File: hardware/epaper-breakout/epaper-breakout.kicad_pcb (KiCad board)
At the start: 2 copper layers, 99.6 x 31.2 mm, 68 parts, among them J1 XF2M-3315-1A, J2 C10418, J3 Conn_02x06_Counter_Clockwise, J4 ED060SC4, Q1 IRLML6402, U1 MCP1700-3302E_SOT23, U2 LT1945, U3 LT1945, U5 ESP32-WROVER, U6 CH330N, U7 LM358, U8 74HC4094-normal, U9 MCP9700AT-ETT

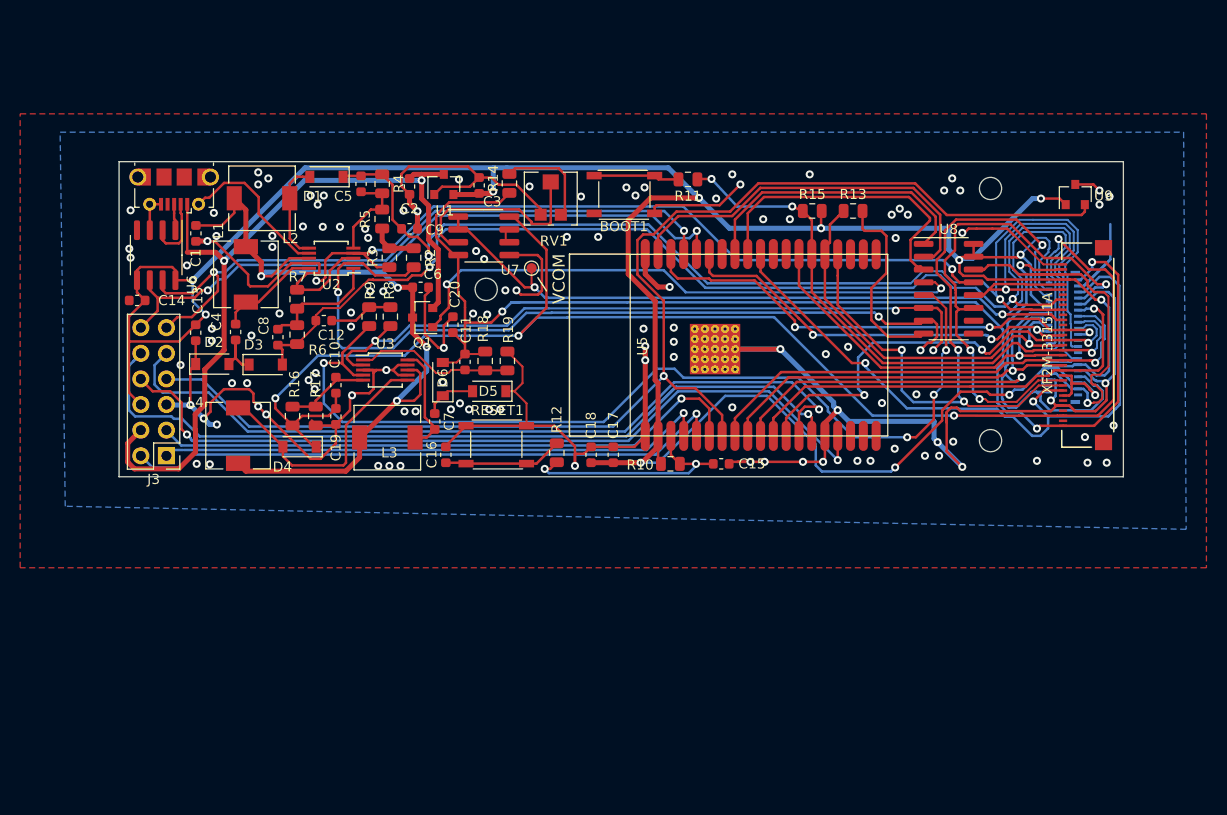
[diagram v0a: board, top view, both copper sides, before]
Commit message: WIP: partial routing
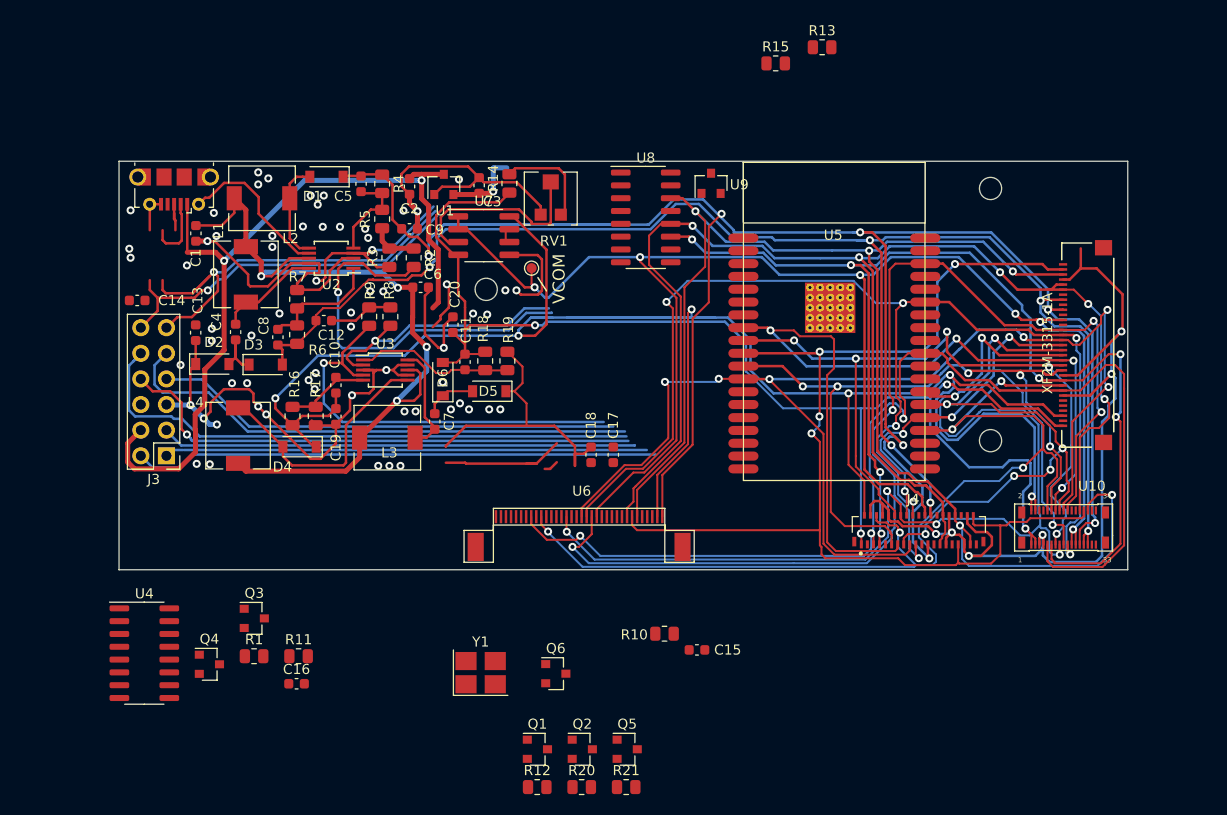
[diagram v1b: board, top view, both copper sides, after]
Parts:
- removed BOOT1: SW2, epaper-breakout:SW_TS-1187A
- removed RESET1: SW1, epaper-breakout:SW_TS-1187A
- added Q2: AO3401A, Package_TO_SOT_SMD:SOT-23, F.Cu at (70.9, 77.8)
- added Q3: MMBT3904, Package_TO_SOT_SMD:SOT-23, F.Cu at (38.4, 64.8)
- added Q4: MMBT3904, Package_TO_SOT_SMD:SOT-23, F.Cu at (34.0, 69.4)
- added Q5: AO3401A, Package_TO_SOT_SMD:SOT-23, F.Cu at (75.4, 77.8)
- added Q6: MMBT3904, Package_TO_SOT_SMD:SOT-23, F.Cu at (68.3, 70.3)
- added R1: 10k, Resistor_SMD:R_0805_2012Metric, F.Cu at (38.4, 68.6)
- added R20: 10k, Resistor_SMD:R_0805_2012Metric, F.Cu at (70.9, 81.5)
- added R21: 10k, Resistor_SMD:R_0805_2012Metric, F.Cu at (75.3, 81.5)
- added U10: ED060SC7, epaper-breakout:AXT334124, F.Cu at (118.6, 57.5)
- added U4: CH340G, Package_SO:SOIC-16_3.9x9.9mm_P1.27mm, F.Cu at (27.5, 68.3)
- added Y1: Crystal_GND2, Crystal:Crystal_SMD_3225-4Pin_3.2x2.5mm_HandSoldering, F.Cu at (60.9, 70.2)
- C13, C14: value 0.1uF -> 10pF
- C15, C16: value 1nF -> 0.1uF
- J4: moved to F.Cu
- Q1: value IRLML6402 -> MMBT3904
- R11: value 470 -> 10k
- R12: value 470 -> 1k
- U6: value CH330N -> ED060XC5; footprint Package_SO:SOIC-8_3.9x4.9mm_P1.27mm -> epaper-breakout:X05A20H34G
- moved R11 61.0 mm to (42.8, 68.6), turned to 0 degrees
- moved U6 49.3 mm to (70.6, 54.7), turned to 0 degrees
- moved Q1 44.3 mm to (66.5, 77.8), turned to 0 degrees
- moved U9 36.1 mm to (83.7, 21.7)
- moved R12 33.2 mm to (66.5, 81.5), turned to 0 degrees
- moved U8 30.9 mm to (77.2, 25.1)
- moved C16 27.1 mm to (42.6, 71.3), turned to 0 degrees
- moved J4 23.9 mm to (104.3, 56.1), turned to 0 degrees
- moved U5 22.8 mm to (95.9, 26.2), turned to 0 degrees
- moved C15 18.6 mm to (82.3, 67.9)
- moved R10 16.9 mm to (79.1, 66.3)
- moved R13 16.5 mm to (94.7, 8.20)
- moved R15 15.1 mm to (90.1, 9.80)
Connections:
- C1 pad 1: EPD_POWER -> SW_VIN
- C13 pad 1: /+3.3V -> Net-(C13-Pad1)
- C14 pad 1: /+3.3V -> GND
- C14 pad 2: GND -> Net-(C14-Pad2)
- C15 pad 1: GND -> /EN
- C15 pad 2: /EN -> GND
- C16 pad 1: GND -> /+3.3V
- C16 pad 2: Net-(C16-Pad2) -> GND
- C6 pad 1: EPD_POWER -> SW_VIN
- J1 pad 11: /+3.3V -> EPD_VDD
- J1 pad 30: /+3.3V -> EPD_VDD
- J1 pad 7: /+3.3V -> EPD_VDD
- J4 pad 10: /+3.3V -> EPD_VDD
- J4 pad 29: /+3.3V -> EPD_VDD
- J4 pad 30: /+3.3V -> EPD_VDD
- J4 pad 35: /+3.3V -> EPD_VDD
- J4 pad 36: /+3.3V -> EPD_VDD
- J4 pad 4: /+3.3V -> EPD_VDD
- J4 pad 8: /+3.3V -> EPD_VDD
- L1 pad 2: EPD_POWER -> SW_VIN
- L2 pad 2: EPD_POWER -> SW_VIN
- L3 pad 2: EPD_POWER -> SW_VIN
- L4 pad 2: EPD_POWER -> SW_VIN
- Q1 pad 1: /~SMPS_CTRL -> Net-(Q1-Pad1)
- Q1 pad 2: 5V -> GND
- Q1 pad 3: EPD_POWER -> Net-(Q1-Pad3)
- R11 pad 1: /EP_D3 -> Net-(Q4-Pad1)
- R11 pad 2: Net-(BOOT1-Pad2) -> /~RTS
- R12 pad 1: /EN -> Net-(Q1-Pad1)
- R12 pad 2: Net-(C16-Pad2) -> /SMPS_CTRL
- U2 pad 8: EPD_POWER -> SW_VIN
- U3 pad 8: EPD_POWER -> SW_VIN
- U6 pad 1: Net-(J2-Pad3) -> /-15V
- U6 pad 2: Net-(J2-Pad2) -> /-20V
- U6 pad 5: /+3.3V -> (no net)
- U6 pad 6: /USB_TXD -> EPD_VDD
- U6 pad 7: /USB_RXD -> GND
- U6 pad 8: /+3.3V -> /EP_CKH
- U8 pad 4: /~SMPS_CTRL -> /SMPS_CTRL
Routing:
- net /+3.3V: track 306.9 -> 8.42 mm, vias 13 -> 1
- net GND: track 368.8 -> 187.1 mm, vias 122 -> 62
- net /EP_STV: track 37.3 -> 139.0 mm, vias 1 -> 5
- net /+22V: track 115.5 -> 210.9 mm, vias 2 -> 7
- net EPD_VDD: track 0.00 -> 94.2 mm, vias 0 -> 6
- net /EP_MODE: track 46.7 -> 138.2 mm, vias 1 -> 5
- net SW_VIN: track 0.00 -> 81.7 mm, vias 0 -> 4
- net EPD_POWER: track 81.7 -> 0.00 mm, vias 4 -> 0
- net /A1: track 126.2 -> 46.3 mm, vias 1 -> 0
- net /EP_D6: track 41.9 -> 118.7 mm, vias 3 -> 6
- net /EP_D5: track 43.6 -> 117.2 mm, vias 3 -> 6
- net /EP_D7: track 48.5 -> 119.5 mm, vias 3 -> 5
- net /EP_D2: track 39.2 -> 109.3 mm, vias 1 -> 6
- net /EP_VCOM: track 95.0 -> 159.7 mm, vias 2 -> 6
- net /EP_OE: track 50.9 -> 114.4 mm, vias 3 -> 7
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- removed copper zone on B.Cu, net GND
- removed copper zone on F.Cu, net GND
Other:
- board size 99.6 x 31.2 mm -> 100 x 40.5 mm
- net class Default: clearance 0.2 -> 0.16
- rule trace_clearance: 0.2 -> 0.16

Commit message: partial routing
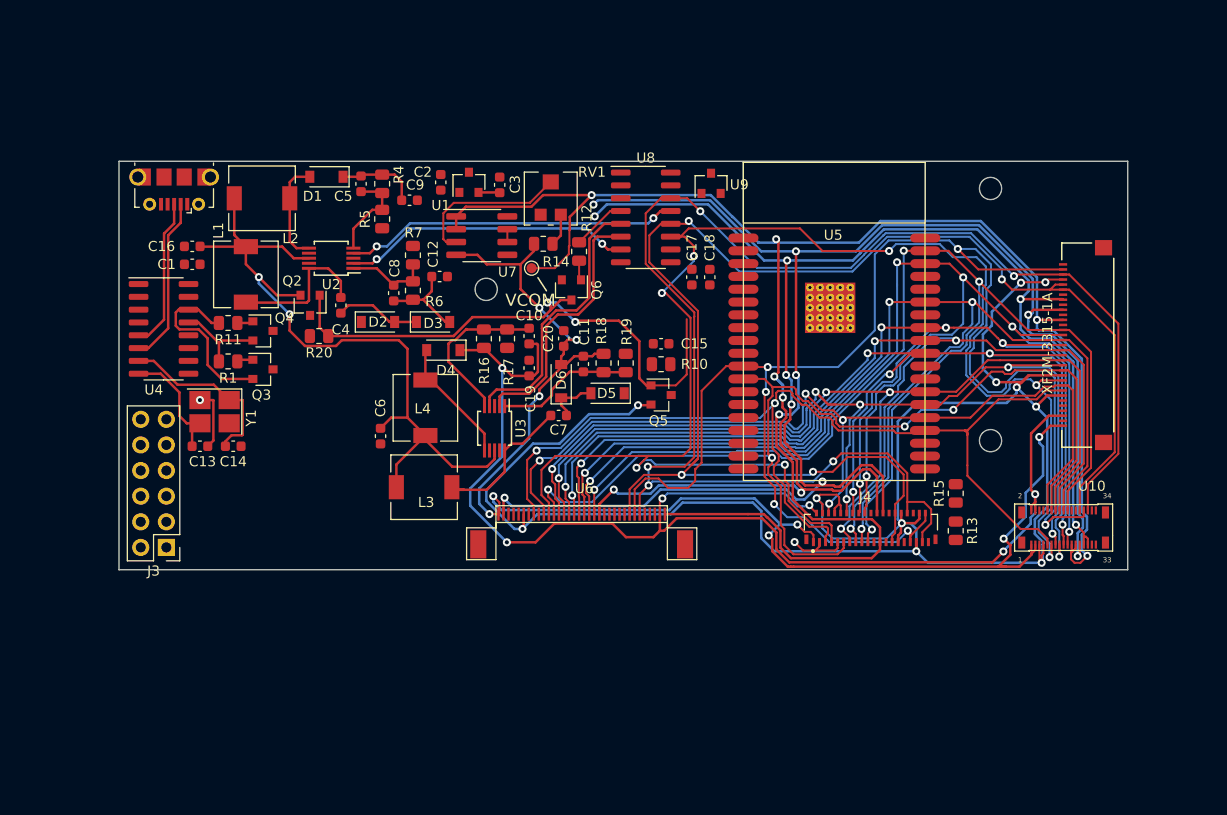
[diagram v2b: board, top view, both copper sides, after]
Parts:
- removed Q1: MMBT3904, Package_TO_SOT_SMD:SOT-23
- removed R2, R21, R3, R8, R9: 10k, Resistor_SMD:R_0805_2012Metric
- moved R12 53.3 mm to (70.6, 28.4), turned to 90 degrees
- moved R20 51.7 mm to (44.8, 36.8), turned to 180 degrees
- moved Q2 51.6 mm to (43.9, 33.8), turned to 270 degrees
- moved R13 49.7 mm to (108.0, 56.1), turned to 270 degrees
- moved R15 46.2 mm to (108.0, 52.4), turned to 90 degrees
- moved C16 42.8 mm to (32.3, 29.7)
- moved Q6 38.1 mm to (69.8, 32.3), turned to 270 degrees
- moved Y1 36.9 mm to (34.5, 44.3), turned to 180 degrees
- moved Q5 35.3 mm to (78.7, 42.7)
- moved R11 33.8 mm to (35.8, 35.5), turned to 180 degrees
- moved Q4 33.5 mm to (39.3, 36.3)
- moved U4 32.2 mm to (29.4, 36.1)
- moved C15 30.6 mm to (78.7, 37.6), turned to 0 degrees
- moved R1 29.3 mm to (35.8, 39.3), turned to 180 degrees
- moved R10 26.7 mm to (78.7, 39.6), turned to 180 degrees
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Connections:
- Q4 pad 3: /EP_D3 -> /EP_D0
- Q5 pad 1: Net-(Q1-Pad3) -> Net-(Q2-Pad1)
- R13 pad 1: /EP_D4 -> /EP_LE
- R15 pad 1: /EP_D3 -> /+3.3V
- R15 pad 2: /+3.3V -> /EP_D0
- U5 pad 10: /EP_CKV -> Net-(U5-Pad10)
- U5 pad 11: /EP_STH -> /EP_CKV
- U5 pad 12: /EP_D5 -> /EP_STH
- U5 pad 23: /EP_LE -> /EP_CKH
- U5 pad 24: /EP_D4 -> /EP_LE
- U5 pad 25: /EP_D3 -> /EP_D0
- U5 pad 26: /EP_D2 -> /EP_D1
- U5 pad 29: /EP_CKH -> /EP_D2
- U5 pad 30: Net-(U5-Pad30) -> /EP_D3
- U5 pad 31: Net-(U5-Pad31) -> /EP_D4
- U5 pad 33: /EP_D6 -> /EP_D5
- U5 pad 36: /EP_D7 -> /EP_D6
- U5 pad 37: Net-(U5-Pad37) -> /EP_D7
- U5 pad 8: /EP_D1 -> Net-(U5-Pad8)
- U5 pad 9: /EP_D0 -> Net-(U5-Pad9)
- U8 pad 1: Net-(U5-Pad31) -> Net-(U5-Pad10)
- U8 pad 2: Net-(U5-Pad37) -> Net-(U5-Pad9)
- U8 pad 3: Net-(U5-Pad30) -> Net-(U5-Pad8)
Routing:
- net GND: track 187.1 -> 12.6 mm, vias 62 -> 2
- net EPD_VDD: track 94.2 -> 188.3 mm, vias 6 -> 11
- net 5V: track 81.2 -> 0.00 mm, vias 2 -> 0
- net /15V: track 198.9 -> 127.1 mm
- net /MISO: track 57.6 -> 0.00 mm
- net /EP_D4: track 54.1 -> 110.9 mm, vias 5 -> 6
- net Net-(Q2-Pad1): track 0.00 -> 56.3 mm, vias 0 -> 2
- net /+22V: track 210.9 -> 157.3 mm, vias 7 -> 6
- net /MOSI: track 52.5 -> 0.00 mm, vias 1 -> 0
- net /SCLK: track 52.1 -> 0.00 mm
- net /SENSOR_VN: track 52.1 -> 0.00 mm
- net /SENSOR_VP: track 47.8 -> 0.00 mm
- net /A0: track 47.0 -> 0.00 mm
- net /A1: track 46.3 -> 0.00 mm
- net /EP_D3: track 60.3 -> 106.0 mm, vias 6 -> 4
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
